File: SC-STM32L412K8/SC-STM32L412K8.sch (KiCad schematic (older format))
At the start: 59 parts, among them J1 usb, J2 +29.6, J3 TxD, J4 RxD, J5 SWDIO, J6 SWCLK, J7 +BAT, J8 SiPM-, J9 BT Status, Q1 IRLML5203, SW1 power, U1 LP2985-3.0, U2 LM2733YMF, U3 LTC4054ES5, U4 LMV7239M5, U5 MCP1700-3002E

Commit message: SC-STM32L412K8/SC-STM32L412K8-rescue.dcm 	SC-STM32L412K8/SC-STM32L412K8-rescue.lib 	SC-STM32L412K8/sym-lib-table
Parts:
- D6: symbol My_Library:STM32L412K8 -> SC-STM32L412K8-rescue:STM32L412K8-My_Library
- J2, J3, J4, J5, J6, J7, J8, J9: symbol My_Library:Conn -> SC-STM32L412K8-rescue:Conn-My_Library
- U4: symbol My_Library:LMV7239M5 -> SC-STM32L412K8-rescue:LMV7239M5-My_Library
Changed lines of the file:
@@
 $EndDescr
 $Comp
-L My_Library:STM32L412K8 D6
+L SC-STM32L412K8-rescue:STM32L412K8-My_Library D6
 U 1 1 60361EE9
 P 7350 4450
@@
 $EndComp
 $Comp
-L My_Library:Conn J5
+L SC-STM32L412K8-rescue:Conn-My_Library J5
 U 1 1 603AE044
 P 6750 5250
@@
 $EndComp
 $Comp
-L My_Library:Conn J6
+L SC-STM32L412K8-rescue:Conn-My_Library J6
 U 1 1 603AE9C5
 P 6750 5350
@@
 $EndComp
 $Comp
-L My_Library:Conn J3
+L SC-STM32L412K8-rescue:Conn-My_Library J3
 U 1 1 603B523F
 P 6750 4850
@@
 $EndComp
 $Comp
-L My_Library:Conn J4
+L SC-STM32L412K8-rescue:Conn-My_Library J4
 U 1 1 603B58EC
 P 6750 4950
@@
 Connection ~ 3850 1450
 $Comp
-L My_Library:Conn J2
+L SC-STM32L412K8-rescue:Conn-My_Library J2
 U 1 1 604E175B
 P 6150 1450
@@
 Connection ~ 7950 3750
 $Comp
-L My_Library:Conn J7
+L SC-STM32L412K8-rescue:Conn-My_Library J7
 U 1 1 60622710
 P 5200 3700
@@
 Connection ~ 5200 3600
 $Comp
-L My_Library:Conn J8
+L SC-STM32L412K8-rescue:Conn-My_Library J8
 U 1 1 606AB650
 P 5250 5050
@@
 $EndComp
 $Comp
-L My_Library:Conn J9
+L SC-STM32L412K8-rescue:Conn-My_Library J9
 U 1 1 6072E770
 P 6750 5450
@@
 	5350 3600 5350 2900
 $Comp
-L My_Library:LMV7239M5 U4
+L SC-STM32L412K8-rescue:LMV7239M5-My_Library U4
 U 1 1 6056F677
 P 6200 5050

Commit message: modified:   SC-STM32L412K8/SC-STM32L412K8-cache.lib 	modified:   SC-STM32L412K8/SC-STM32L412K8.kicad_pcb 	modified:   SC-STM32L412K8/SC-STM32L412K8.kicad_pcb-bak 	modified:   SC-STM32L412K8/SC-STM32L412K8.net 	modified:   SC-STM32L412K8/SC-STM32L412K8.sch 	modified:   SC-STM32L412K8/SC-STM32L412K8.sch-bak
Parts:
- added J?: PWM, My-library:SMD-CONN, symbol SC-STM32L412K8-rescue:Conn-My_Library-SC-STM32L412K8-rescue
- D6: symbol SC-STM32L412K8-rescue:STM32L412K8-My_Library -> SC-STM32L412K8-rescue:STM32L412K8-My_Library-SC-STM32L412K8-rescue
- J2, J3, J4, J5, J6, J7, J8, J9: symbol SC-STM32L412K8-rescue:Conn-My_Library -> SC-STM32L412K8-rescue:Conn-My_Library-SC-STM32L412K8-rescue
- U4: symbol SC-STM32L412K8-rescue:LMV7239M5-My_Library -> SC-STM32L412K8-rescue:LMV7239M5-My_Library-SC-STM32L412K8-rescue
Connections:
- net at D6.22 (PA12): now also J?.1 (Pin_1)
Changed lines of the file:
@@
 $EndDescr
 $Comp
-L SC-STM32L412K8-rescue:STM32L412K8-My_Library D6
+L SC-STM32L412K8-rescue:STM32L412K8-My_Library-SC-STM32L412K8-rescue D6
 U 1 1 60361EE9
 P 7350 4450
@@
 $EndComp
 $Comp
-L SC-STM32L412K8-rescue:Conn-My_Library J5
+L SC-STM32L412K8-rescue:Conn-My_Library-SC-STM32L412K8-rescue J5
 U 1 1 603AE044
 P 6750 5250
@@
 $EndComp
 $Comp
-L SC-STM32L412K8-rescue:Conn-My_Library J6
+L SC-STM32L412K8-rescue:Conn-My_Library-SC-STM32L412K8-rescue J6
 U 1 1 603AE9C5
 P 6750 5350
@@
 $EndComp
 $Comp
-L SC-STM32L412K8-rescue:Conn-My_Library J3
+L SC-STM32L412K8-rescue:Conn-My_Library-SC-STM32L412K8-rescue J3
 U 1 1 603B523F
 P 6750 4850
@@
 $EndComp
 $Comp
-L SC-STM32L412K8-rescue:Conn-My_Library J4
+L SC-STM32L412K8-rescue:Conn-My_Library-SC-STM32L412K8-rescue J4
 U 1 1 603B58EC
 P 6750 4950
@@
 Connection ~ 3850 1450
 $Comp
-L SC-STM32L412K8-rescue:Conn-My_Library J2
+L SC-STM32L412K8-rescue:Conn-My_Library-SC-STM32L412K8-rescue J2
 U 1 1 604E175B
 P 6150 1450
@@
 Connection ~ 7950 3750
 $Comp
-L SC-STM32L412K8-rescue:Conn-My_Library J7
+L SC-STM32L412K8-rescue:Conn-My_Library-SC-STM32L412K8-rescue J7
 U 1 1 60622710
 P 5200 3700
@@
 Connection ~ 5200 3600
 $Comp
-L SC-STM32L412K8-rescue:Conn-My_Library J8
+L SC-STM32L412K8-rescue:Conn-My_Library-SC-STM32L412K8-rescue J8
 U 1 1 606AB650
 P 5250 5050
@@
 $EndComp
 $Comp
-L SC-STM32L412K8-rescue:Conn-My_Library J9
+L SC-STM32L412K8-rescue:Conn-My_Library-SC-STM32L412K8-rescue J9
 U 1 1 6072E770
 P 6750 5450
@@
 	5350 3600 5350 2900
 $Comp
-L SC-STM32L412K8-rescue:LMV7239M5-My_Library U4
+L SC-STM32L412K8-rescue:LMV7239M5-My_Library-SC-STM32L412K8-rescue U4
 U 1 1 6056F677
 P 6200 5050
@@
 Wire Wire Line
 	6300 4500 6150 4500
+$Comp
+L SC-STM32L412K8-rescue:Conn-My_Library-SC-STM32L412K8-rescue J?
+U 1 1 604B8416
+P 6750 5150
+F 0 "J?" H 6692 4925 50  0001 C CNN
+F 1 "PWM" H 6900 5150 50  0000 C CNN
+F 2 "My-library:SMD-CONN" H 6750 5150 50  0001 C CNN
+F 3 "~" H 6750 5150 50  0001 C CNN
+	1    6750 5150
+	-1   0    0    1
+$EndComp
 $EndSCHEMATC

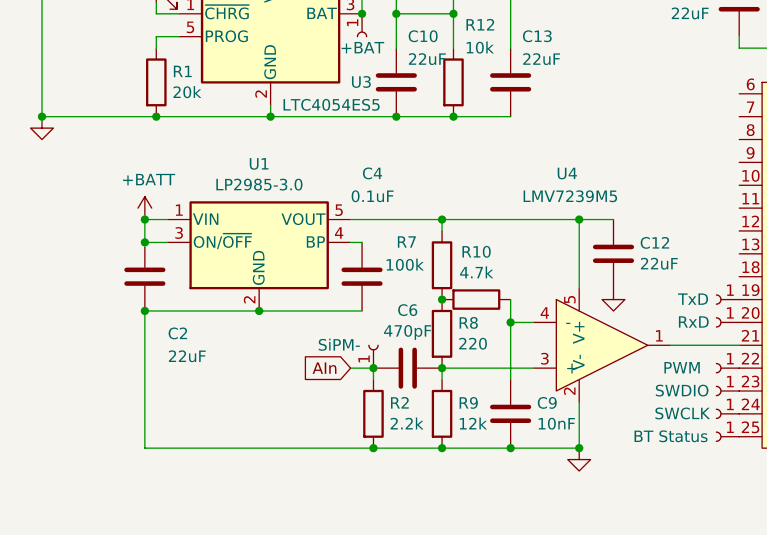
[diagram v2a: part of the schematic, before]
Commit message: modified:   SC-STM32L412K8/SC-STM32L412K8.kicad_pcb 	modified:   SC-STM32L412K8/SC-STM32L412K8.kicad_pcb-bak 	modified:   SC-STM32L412K8/SC-STM32L412K8.sch 	modified:   SC-STM32L412K8/SC-STM32L412K8.sch-bak
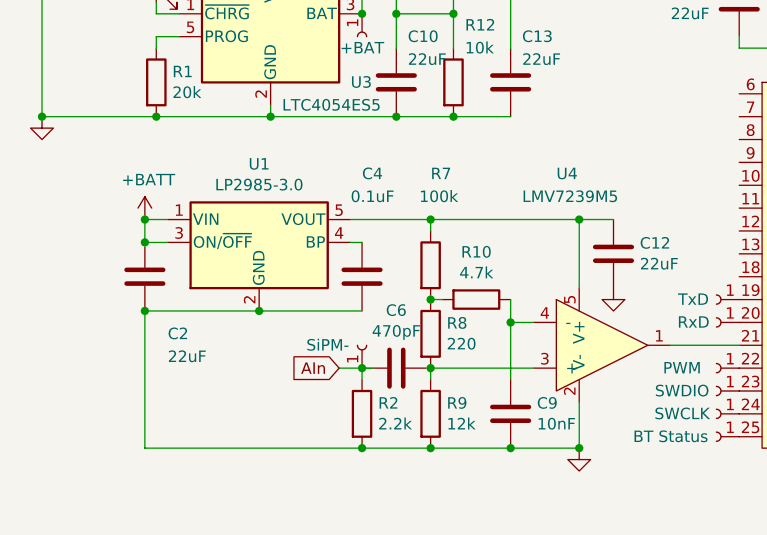
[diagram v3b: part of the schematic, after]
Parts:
- gave numbers to parts that had none: 1
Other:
- moved on the sheet: C6, R2, R7, R8, R9
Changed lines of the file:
@@
 L Device:R R7
 U 1 1 6036B072
-P 5550 4700
-F 0 "R7" H 5350 4800 50  0000 L CNN
-F 1 "100k" H 5300 4700 50  0000 L CNN
-F 2 "Resistor_SMD:R_0603_1608Metric" V 5480 4700 50  0001 C CNN
-F 3 "~" H 5550 4700 50  0001 C CNN
-	1    5550 4700
+P 5500 4700
+F 0 "R7" H 5500 5100 50  0000 L CNN
+F 1 "100k" H 5450 5000 50  0000 L CNN
+F 2 "Resistor_SMD:R_0603_1608Metric" V 5430 4700 50  0001 C CNN
+F 3 "~" H 5500 4700 50  0001 C CNN
+	1    5500 4700
 	1    0    0    -1
 $EndComp
@@
 L Device:R R8
 U 1 1 6036B7B6
-P 5550 5000
-F 0 "R8" H 5620 5046 50  0000 L CNN
-F 1 "220" H 5620 4955 50  0000 L CNN
-F 2 "Resistor_SMD:R_0603_1608Metric" V 5480 5000 50  0001 C CNN
-F 3 "~" H 5550 5000 50  0001 C CNN
-	1    5550 5000
+P 5500 5000
+F 0 "R8" H 5570 5046 50  0000 L CNN
+F 1 "220" H 5570 4955 50  0000 L CNN
+F 2 "Resistor_SMD:R_0603_1608Metric" V 5430 5000 50  0001 C CNN
+F 3 "~" H 5500 5000 50  0001 C CNN
+	1    5500 5000
 	1    0    0    -1
 $EndComp
@@
 L Device:R R9
 U 1 1 6036BC49
-P 5550 5350
-F 0 "R9" H 5620 5396 50  0000 L CNN
-F 1 "12k" H 5620 5305 50  0000 L CNN
-F 2 "Resistor_SMD:R_0603_1608Metric" V 5480 5350 50  0001 C CNN
-F 3 "~" H 5550 5350 50  0001 C CNN
-	1    5550 5350
+P 5500 5350
+F 0 "R9" H 5570 5396 50  0000 L CNN
+F 1 "12k" H 5570 5305 50  0000 L CNN
+F 2 "Resistor_SMD:R_0603_1608Metric" V 5430 5350 50  0001 C CNN
+F 3 "~" H 5500 5350 50  0001 C CNN
+	1    5500 5350
 	1    0    0    -1
 $EndComp
@@
 L Device:C C6
 U 1 1 6036D36F
-P 5400 5150
-F 0 "C6" V 5148 5150 50  0000 C CNN
-F 1 "470pF" V 5239 5150 50  0000 C CNN
-F 2 "Capacitor_SMD:C_0603_1608Metric" H 5438 5000 50  0001 C CNN
-F 3 "~" H 5400 5150 50  0001 C CNN
-	1    5400 5150
+P 5350 5150
+F 0 "C6" V 5098 5150 50  0000 C CNN
+F 1 "470pF" V 5189 5150 50  0000 C CNN
+F 2 "Capacitor_SMD:C_0603_1608Metric" H 5388 5000 50  0001 C CNN
+F 3 "~" H 5350 5150 50  0001 C CNN
+	1    5350 5150
 	0    1    1    0
 $EndComp
@@
 L Device:R R2
 U 1 1 6036DAFE
-P 5250 5350
-F 0 "R2" H 5320 5396 50  0000 L CNN
-F 1 "2.2k" H 5320 5305 50  0000 L CNN
-F 2 "Resistor_SMD:R_0603_1608Metric" V 5180 5350 50  0001 C CNN
-F 3 "~" H 5250 5350 50  0001 C CNN
-	1    5250 5350
+P 5200 5350
+F 0 "R2" H 5270 5396 50  0000 L CNN
+F 1 "2.2k" H 5270 5305 50  0000 L CNN
+F 2 "Resistor_SMD:R_0603_1608Metric" V 5130 5350 50  0001 C CNN
+F 3 "~" H 5200 5350 50  0001 C CNN
+	1    5200 5350
 	1    0    0    -1
 $EndComp
@@
 Text GLabel 7950 4300 2    50   Input ~ 0
 AIn
-Text GLabel 5150 5150 0    50   Input ~ 0
+Text GLabel 5100 5150 0    50   Input ~ 0
 AIn
 $Comp
@@
 L SC-STM32L412K8-rescue:Conn-My_Library-SC-STM32L412K8-rescue J8
 U 1 1 606AB650
-P 5250 5050
-F 0 "J8" H 5192 4825 50  0001 C CNN
-F 1 "SiPM-" V 5250 5200 50  0000 C CNN
-F 2 "My-library:SMD-CONN" H 5250 5050 50  0001 C CNN
-F 3 "~" H 5250 5050 50  0001 C CNN
-	1    5250 5050
+P 5200 5050
+F 0 "J8" H 5142 4825 50  0001 C CNN
+F 1 "SiPM-" V 5200 5200 50  0000 C CNN
+F 2 "My-library:SMD-CONN" H 5200 5050 50  0001 C CNN
+F 3 "~" H 5200 5050 50  0001 C CNN
+	1    5200 5050
 	0    -1   -1   0
 $EndComp
@@
 Wire Wire Line
 	7500 3400 7950 3400
-Connection ~ 5550 4850
-Wire Wire Line
-	5550 4550 5550 4500
-Wire Wire Line
-	5550 4500 6150 4500
 Wire Wire Line
 	6150 5300 6150 5500
@@
 	6150 5500 5850 5500
 Connection ~ 6150 5500
-Connection ~ 5550 5500
-Wire Wire Line
-	5550 5500 5250 5500
 Connection ~ 5850 5500
-Wire Wire Line
-	5850 5500 5550 5500
-Wire Wire Line
-	5150 5150 5250 5150
-Wire Wire Line
-	5250 5150 5250 5200
-Connection ~ 5250 5150
-Wire Wire Line
-	5550 5200 5550 5150
-Wire Wire Line
-	5550 5150 5950 5150
-Connection ~ 5550 5150
 Wire Wire Line
 	5850 5200 5850 4950
@@
 	5200 4900 4750 4900
 Wire Wire Line
-	5150 4500 5550 4500
-Connection ~ 5550 4500
-Wire Wire Line
-	4250 5500 5250 5500
-Connection ~ 5250 5500
+	5150 4500 5500 4500
+Wire Wire Line
+	4250 5500 5200 5500
 Wire Wire Line
 	6550 5050 6850 5050
@@
 	6300 4500 6150 4500
 $Comp
-L SC-STM32L412K8-rescue:Conn-My_Library-SC-STM32L412K8-rescue J?
+L SC-STM32L412K8-rescue:Conn-My_Library-SC-STM32L412K8-rescue J10
 U 1 1 604B8416
 P 6750 5150
-F 0 "J?" H 6692 4925 50  0001 C CNN
+F 0 "J10" H 6692 4925 50  0001 C CNN
 F 1 "PWM" H 6900 5150 50  0000 C CNN
 F 2 "My-library:SMD-CONN" H 6750 5150 50  0001 C CNN
@@
 	-1   0    0    1
 $EndComp
+Connection ~ 5200 5150
+Wire Wire Line
+	5200 5150 5250 5150
+Connection ~ 5200 5500
+Connection ~ 5500 5500
+Wire Wire Line
+	5550 4850 5500 4850
+Wire Wire Line
+	5500 5500 5850 5500
+Wire Wire Line
+	5200 5500 5500 5500
+Connection ~ 5500 4850
+Wire Wire Line
+	5500 4550 5500 4500
+Connection ~ 5500 4500
+Wire Wire Line
+	5500 4500 6150 4500
+Wire Wire Line
+	5100 5150 5200 5150
+Wire Wire Line
+	5200 5150 5200 5200
+Wire Wire Line
+	5500 5200 5500 5150
+Connection ~ 5500 5150
+Wire Wire Line
+	5500 5150 5950 5150
 $EndSCHEMATC
